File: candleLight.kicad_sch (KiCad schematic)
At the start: 3 parts

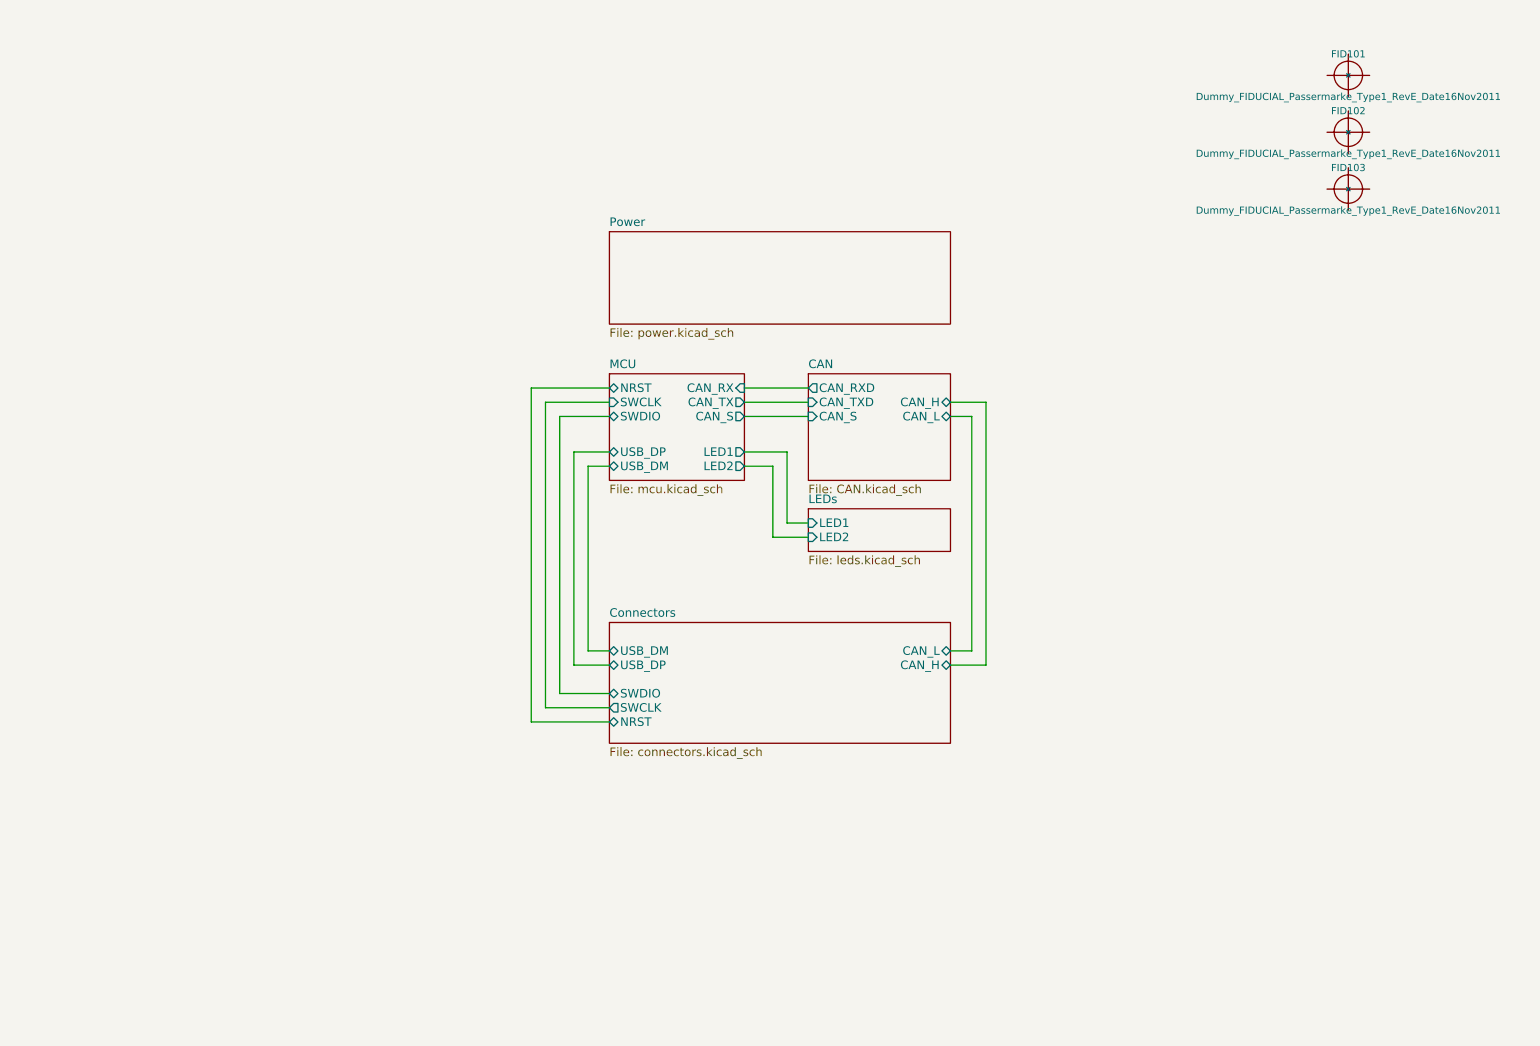
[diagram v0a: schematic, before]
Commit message: schematic
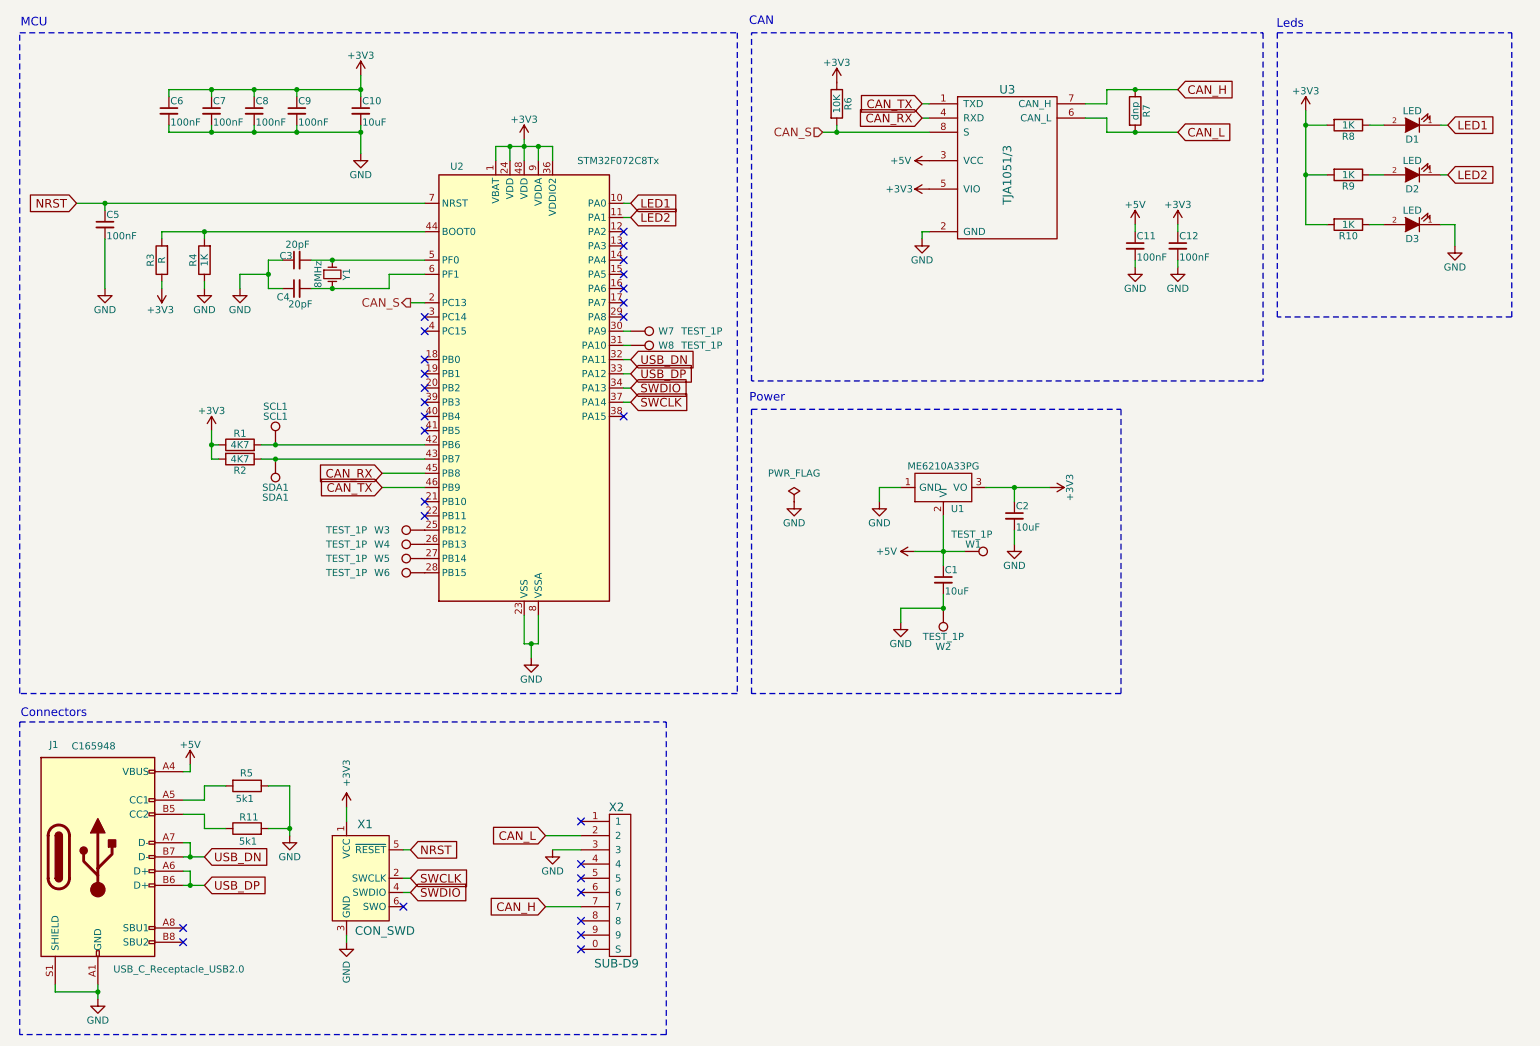
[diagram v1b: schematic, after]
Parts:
- removed FID101, FID102, FID103: Dummy_FIDUCIAL_Passermarke_Type1_RevE_Date16Nov20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, Fiducials:Fiducial_1mm_Dia_2.54mm_Outer_CopperTop, symbol candleLight-rescue:Dummy_FIDUCIAL_Passermarke_Type1_RevE_Date16Nov2011
- added C1, C10, C2: 10uF, Capacitor_SMD:C_0805_2012Metric, symbol candleLight-rescue:C_Small
- added C11, C12, C5, C6, C7, C8, C9: 100nF, Capacitor_SMD:C_0603_1608Metric, symbol candleLight-rescue:C_Small
- added C3, C4: 20pF, Capacitor_SMD:C_0603_1608Metric, symbol candleLight-rescue:C_Small
- added D1, D2, D3: LED, LED_SMD:LED_0603_1608Metric, symbol candleLight-rescue:LED
- added J1: USB_C_Receptacle_USB2.0, stm32world:USB_C_Receptacle_HRO_TYPE-C-31-M-12, symbol stm32world:USB_C_Receptacle_USB2.0
- added R1, R2: 4K7, Resistor_SMD:R_0603_1608Metric, symbol candleLight-rescue:R
- added R10, R4, R8, R9: 1K, Resistor_SMD:R_0603_1608Metric, symbol candleLight-rescue:R
- added R11, R5: 5k1, Resistor_SMD:R_0603_1608Metric, symbol Device:R
- added R3: R, Resistor_SMD:R_0805_2012Metric, symbol candleLight-rescue:R
- added R6: 10K, Resistor_SMD:R_0603_1608Metric, symbol candleLight-rescue:R
- added R7: dnp, Resistor_SMD:R_0805_2012Metric, symbol candleLight-rescue:R
- added SCL1: SCL1, Measurement_Points:Measurement_Point_Round-SMD-Pad_Small, symbol candleLight-rescue:TEST_1P
- added SDA1: SDA1, Measurement_Points:Measurement_Point_Round-SMD-Pad_Small, symbol candleLight-rescue:TEST_1P
- added U1: ME6210A33PG, Package_TO_SOT_SMD:SOT-89-3, symbol candleLight-rescue:MCP1754ST-3302E/MB
- added U2: STM32F072C8Tx, Package_QFP:LQFP-48_7x7mm_P0.5mm, symbol MCU_ST_STM32F0:STM32F072C8Tx
- added U3: TJA1051/3, Package_SO:SOIC-8_3.9x4.9mm_P1.27mm, symbol candleLight-rescue:TJA1051/3
- added W1, W2: TEST_1P, Measurement_Points:Measurement_Point_Round-SMD-Pad_Big, symbol candleLight-rescue:TEST_1P
- added W3, W4, W5, W6, W7, W8: TEST_1P, Measurement_Points:Measurement_Point_Round-SMD-Pad_Small, symbol candleLight-rescue:TEST_1P
- added X1: CON_SWD, Connector:Tag-Connect_TC2030-IDC-NL_2x03_P1.27mm_Vertical, symbol Connector:Conn_ARM_SWD_TagConnect_TC2030-NL
- added X2: SUB-D9, Connect:DB9M_CI, symbol candleLight-rescue:SUB-D9
- added Y1: 8MHz, Crystal:Crystal_SMD_Abracon_ABM3-2Pin_5.0x3.2mm, symbol candleLight-rescue:Crystal_Small
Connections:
- new net: D1.2 (A), R8.1
- new net: R1.2, SCL1.1, U2.42 (PB6)
- new net: J1.A5 (CC1), R5.2
- new net: J1.B5 (CC2), R11.1
- new net: U2.27 (PB14), W5.1
- new net: R2.1, SDA1.1, U2.43 (PB7)
- new net: U2.25 (PB12), W3.1
- new net: R3.2, R4.2, U2.44 (BOOT0)
- new net: U2.30 (PA9), W7.1
- new net: D3.2 (A), R10.1
- new net: U2.26 (PB13), W4.1
- new net: C3.2, U2.5 (PF0), Y1.1
- new net: C4.2, U2.6 (PF1), Y1.2
- new net: U2.28 (PB15), W6.1
- new net: U2.31 (PA10), W8.1
- new net: D2.2 (A), R9.1
- new net +3V3: C10.1, C12.1, C2.1, C6.1, C7.1, C8.1, C9.1, R1.1, R10.2, R2.2, R3.1, R6.1, R8.2, R9.2, U1.3 (VO), U2.1 (VBAT), U2.24 (VDD), U2.36 (VDDIO2), U2.48 (VDD), U2.9 (VDDA), U3.5 (VIO), X1.1 (VCC)
- new net +5V: C1.1, C11.1, J1.A4 (VBUS), J1.A9 (VBUS), J1.B4 (VBUS), J1.B9 (VBUS), U1.2 (VI), U3.3 (VCC), W1.1
- new net CAN_H: R7.1, U3.7 (CAN_H), X2.7
- new net CAN_L: R7.2, U3.6 (CAN_L), X2.2
- new net CAN_RX: U2.45 (PB8), U3.4 (RXD)
- new net CAN_S: R6.2, U2.2 (PC13), U3.8 (S)
- new net CAN_TX: U2.46 (PB9), U3.1 (TXD)
- new net GND: C1.2, C10.2, C11.2, C12.2, C2.2, C3.1, C4.1, C5.2, C6.2, C7.2, C8.2, C9.2, D3.1 (K), J1.A1 (GND), J1.A12 (GND), J1.B1 (GND), J1.B12 (GND), J1.S1 (SHIELD), R11.2, R4.1, R5.1, U1.1 (GND), U2.23 (VSS), U2.35 (VSS), U2.47 (VSS), U2.8 (VSSA), U3.2 (GND), W2.1, X1.3 (GND), X2.3
- new net LED1: D1.1 (K), U2.10 (PA0)
- new net LED2: D2.1 (K), U2.11 (PA1)
- new net NRST: C5.1, U2.7 (NRST), X1.5 (~{RESET})
- new net SWCLK: U2.37 (PA14), X1.2 (SWCLK)
- new net SWDIO: U2.34 (PA13), X1.4 (SWDIO)
- new net USB_DN: J1.A7 (D-), J1.B7 (D-), U2.32 (PA11)
- new net USB_DP: J1.A6 (D+), J1.B6 (D+), U2.33 (PA12)
- no-connect marks 0 -> 28
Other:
- removed sheet CAN
- removed sheet Connectors
- removed sheet LEDs
- removed sheet MCU
- removed sheet Power
- note added: "CAN"
- note added: "Connectors"
- note added: "Leds"
- note added: "MCU"
- note added: "Power"
- title: (none) -> canleLight
